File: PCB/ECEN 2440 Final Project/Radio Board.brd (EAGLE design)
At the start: 58.4 x 38.1 mm, 27 parts

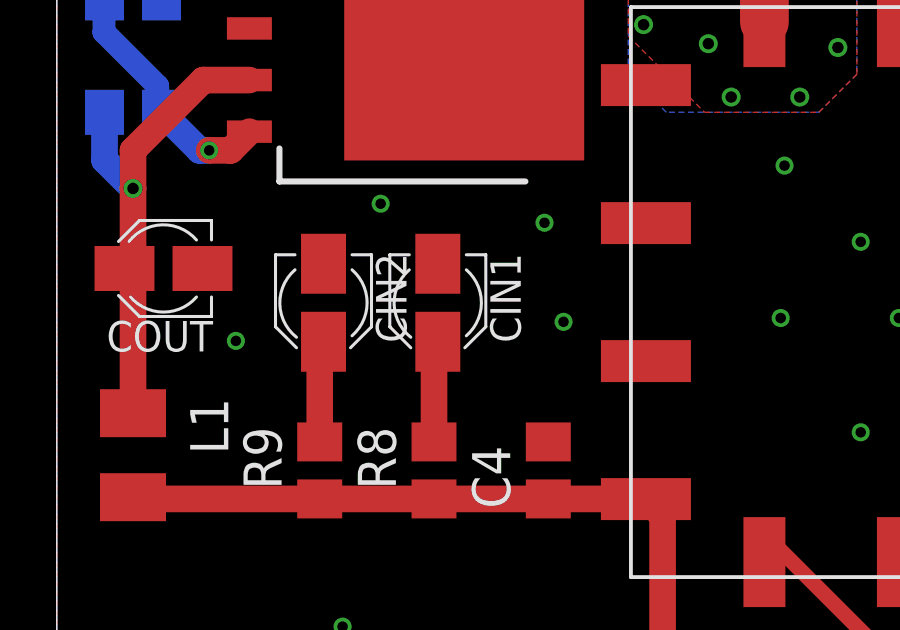
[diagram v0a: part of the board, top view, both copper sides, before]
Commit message: naming
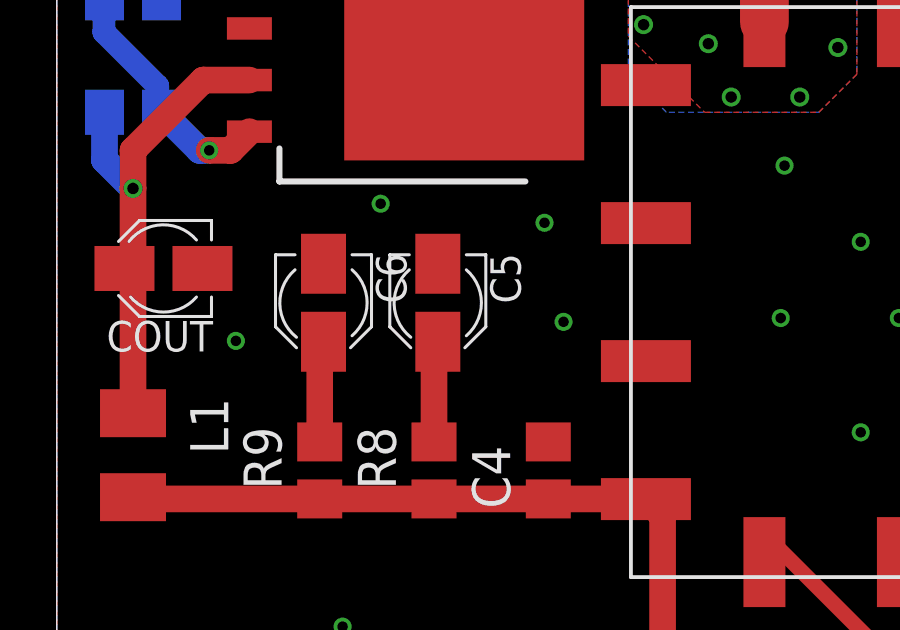
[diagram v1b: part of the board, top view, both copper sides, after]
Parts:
- C1, C2, C3: value 500n -> (none)
- R1, R2, R3: value 100R -> 0R
- renumbered CIN1 to C5, CIN2 to C6
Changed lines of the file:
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@@
 <setting verticaltext="up"/>
 </settings>
-<grid distance="0.05" unitdist="inch" unit="mil" style="lines" multiple="1" display="yes" altdistance="5" altunitdist="mil" altunit="inch"/>
+<grid distance="0.05" unitdist="inch" unit="mm" style="lines" multiple="1" display="yes" altdistance="5" altunitdist="mil" altunit="inch"/>
 <layers>
 <layer number="1" name="Top" color="4" fill="1" visible="yes" active="yes"/>
@@
 </autorouter>
 <elements>
-<element name="C1" library="rcl" library_urn="urn:adsk.eagle:library:334" package="C0805" package3d_urn="urn:adsk.eagle:package:23617/2" value="500n" x="34.544" y="12.319" smashed="yes" rot="MR0">
+<element name="C1" library="rcl" library_urn="urn:adsk.eagle:library:334" package="C0805" package3d_urn="urn:adsk.eagle:package:23617/2" value="" x="34.544" y="12.319" smashed="yes" rot="MR0">
 <attribute name="NAME" x="35.814" y="13.589" size="1.27" layer="26" rot="MR0"/>
 <attribute name="POPULARITY" value="63" x="-2.286" y="-28.321" size="1.778" layer="28" rot="MR0" display="off"/>
@@
 <attribute name="VALUE" x="35.814" y="9.779" size="1.27" layer="28" rot="MR0"/>
 </element>
-<element name="C2" library="rcl" library_urn="urn:adsk.eagle:library:334" package="C0805" package3d_urn="urn:adsk.eagle:package:23617/2" value="500n" x="35.179" y="17.526" smashed="yes" rot="MR0">
+<element name="C2" library="rcl" library_urn="urn:adsk.eagle:library:334" package="C0805" package3d_urn="urn:adsk.eagle:package:23617/2" value="" x="35.179" y="17.526" smashed="yes" rot="MR0">
 <attribute name="NAME" x="36.449" y="18.796" size="1.27" layer="26" rot="MR0"/>
 <attribute name="POPULARITY" value="63" x="-8.001" y="-23.114" size="1.778" layer="28" rot="MR0" display="off"/>
@@
 <attribute name="VALUE" x="36.449" y="14.986" size="1.27" layer="28" rot="MR0"/>
 </element>
-<element name="C3" library="rcl" library_urn="urn:adsk.eagle:library:334" package="C0805" package3d_urn="urn:adsk.eagle:package:23617/2" value="500n" x="34.925" y="22.225" smashed="yes" rot="MR0">
+<element name="C3" library="rcl" library_urn="urn:adsk.eagle:library:334" package="C0805" package3d_urn="urn:adsk.eagle:package:23617/2" value="" x="34.925" y="22.225" smashed="yes" rot="MR0">
 <attribute name="NAME" x="36.195" y="23.495" size="1.27" layer="26" rot="MR0"/>
 <attribute name="POPULARITY" value="63" x="18.415" y="-24.765" size="1.778" layer="28" rot="MR0" display="off"/>
@@
 <attribute name="VALUE" x="45.72" y="6.35" size="1.27" layer="27" rot="R180"/>
 </element>
-<element name="R1" library="rcl" library_urn="urn:adsk.eagle:library:334" package="R0805" package3d_urn="urn:adsk.eagle:package:23553/2" value="100R" x="38.735" y="11.43" smashed="yes" rot="MR90">
+<element name="R1" library="rcl" library_urn="urn:adsk.eagle:library:334" package="R0805" package3d_urn="urn:adsk.eagle:package:23553/2" value="0R" x="38.735" y="11.43" smashed="yes" rot="MR90">
 <attribute name="NAME" x="40.005" y="10.795" size="1.27" layer="26" rot="MR90"/>
 <attribute name="POPULARITY" value="85" x="-1.905" y="29.21" size="1.778" layer="28" rot="MR90" display="off"/>
@@
 <attribute name="VALUE" x="36.195" y="10.795" size="1.27" layer="28" rot="MR90"/>
 </element>
-<element name="R2" library="rcl" library_urn="urn:adsk.eagle:library:334" package="R0805" package3d_urn="urn:adsk.eagle:package:23553/2" value="100R" x="38.735" y="16.51" smashed="yes" rot="MR90">
+<element name="R2" library="rcl" library_urn="urn:adsk.eagle:library:334" package="R0805" package3d_urn="urn:adsk.eagle:package:23553/2" value="0R" x="38.735" y="16.51" smashed="yes" rot="MR90">
 <attribute name="NAME" x="40.005" y="15.875" size="1.27" layer="26" rot="MR90"/>
 <attribute name="POPULARITY" value="85" x="-1.905" y="40.64" size="1.778" layer="28" rot="MR90" display="off"/>
@@
 <attribute name="VALUE" x="36.195" y="15.875" size="1.27" layer="28" rot="MR90"/>
 </element>
-<element name="R3" library="rcl" library_urn="urn:adsk.eagle:library:334" package="R0805" package3d_urn="urn:adsk.eagle:package:23553/2" value="100R" x="38.735" y="21.59" smashed="yes" rot="MR90">
+<element name="R3" library="rcl" library_urn="urn:adsk.eagle:library:334" package="R0805" package3d_urn="urn:adsk.eagle:package:23553/2" value="0R" x="38.735" y="21.59" smashed="yes" rot="MR90">
 <attribute name="NAME" x="40.005" y="20.955" size="1.27" layer="26" rot="MR90"/>
 <attribute name="POPULARITY" value="85" x="-1.905" y="52.07" size="1.778" layer="28" rot="MR90" display="off"/>
@@
 <attribute name="VALUE" x="11.303" y="10.287" size="1.27" layer="27" rot="R90"/>
 </element>
-<element name="CIN1" library="rcl" library_urn="urn:adsk.eagle:library:334" package="PANASONIC_A" package3d_urn="urn:adsk.eagle:package:23418/2" value="" x="12.7" y="16.51" smashed="yes" rot="R270">
+<element name="C5" library="rcl" library_urn="urn:adsk.eagle:library:334" package="PANASONIC_A" package3d_urn="urn:adsk.eagle:package:23418/2" value="" x="12.7" y="16.51" smashed="yes" rot="R270">
 <attribute name="NAME" x="14.45" y="18.16" size="1.016" layer="25" rot="R270"/>
 <attribute name="POPULARITY" value="1" x="12.7" y="16.51" size="1.778" layer="27" rot="R270" display="off"/>
@@
 <attribute name="VALUE" x="9.875" y="18.16" size="1.016" layer="27" rot="R270"/>
 </element>
-<element name="CIN2" library="rcl" library_urn="urn:adsk.eagle:library:334" package="PANASONIC_A" package3d_urn="urn:adsk.eagle:package:23418/2" value="" x="8.89" y="16.51" smashed="yes" rot="R270">
+<element name="C6" library="rcl" library_urn="urn:adsk.eagle:library:334" package="PANASONIC_A" package3d_urn="urn:adsk.eagle:package:23418/2" value="" x="8.89" y="16.51" smashed="yes" rot="R270">
 <attribute name="NAME" x="10.64" y="18.16" size="1.016" layer="25" rot="R270"/>
 <attribute name="POPULARITY" value="1" x="8.89" y="16.51" size="1.778" layer="27" rot="R270" display="off"/>
@@
 <contactref element="COUT" pad="-"/>
 <contactref element="4VPWR" pad="2"/>
-<contactref element="CIN2" pad="-"/>
-<contactref element="CIN1" pad="-"/>
+<contactref element="C6" pad="-"/>
+<contactref element="C5" pad="-"/>
 <contactref element="C4" pad="2"/>
 <via x="10.16" y="36.83" extent="1-16" drill="0.35"/>
@@
 <signal name="N$8">
 <contactref element="R9" pad="2"/>
-<contactref element="CIN2" pad="+"/>
+<contactref element="C6" pad="+"/>
 <wire x1="8.763" y1="15.083" x2="8.89" y2="15.21" width="0.889" layer="1"/>
 <wire x1="8.763" y1="15.083" x2="8.763" y2="11.872" width="0.889" layer="1"/>
@@
 <signal name="N$9">
 <contactref element="R8" pad="2"/>
-<contactref element="CIN1" pad="+"/>
+<contactref element="C5" pad="+"/>
 <wire x1="12.573" y1="15.083" x2="12.7" y2="15.21" width="0.889" layer="1"/>
 <wire x1="12.573" y1="15.083" x2="12.573" y2="11.872" width="0.889" layer="1"/>
